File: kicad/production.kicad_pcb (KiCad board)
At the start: 2 copper layers, 76.2 x 78.7 mm, 54 parts, among them J1 ZX62R-B-5P, P1 CONN, SW1 RESET, SW2 IO0, U1 ESP-WROOM-32, U2 NJM2884, U3 FT231XS

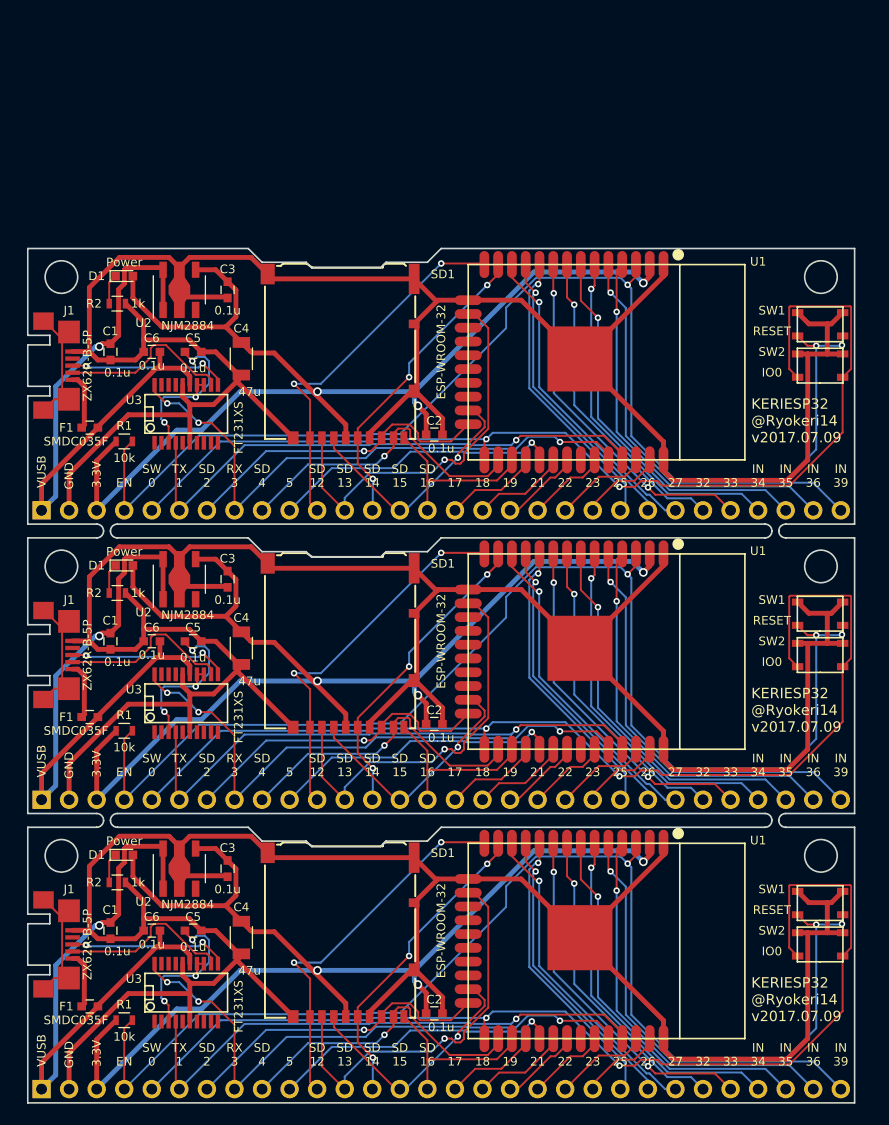
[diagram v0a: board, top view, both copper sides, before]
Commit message: 4枚面付け基板作成
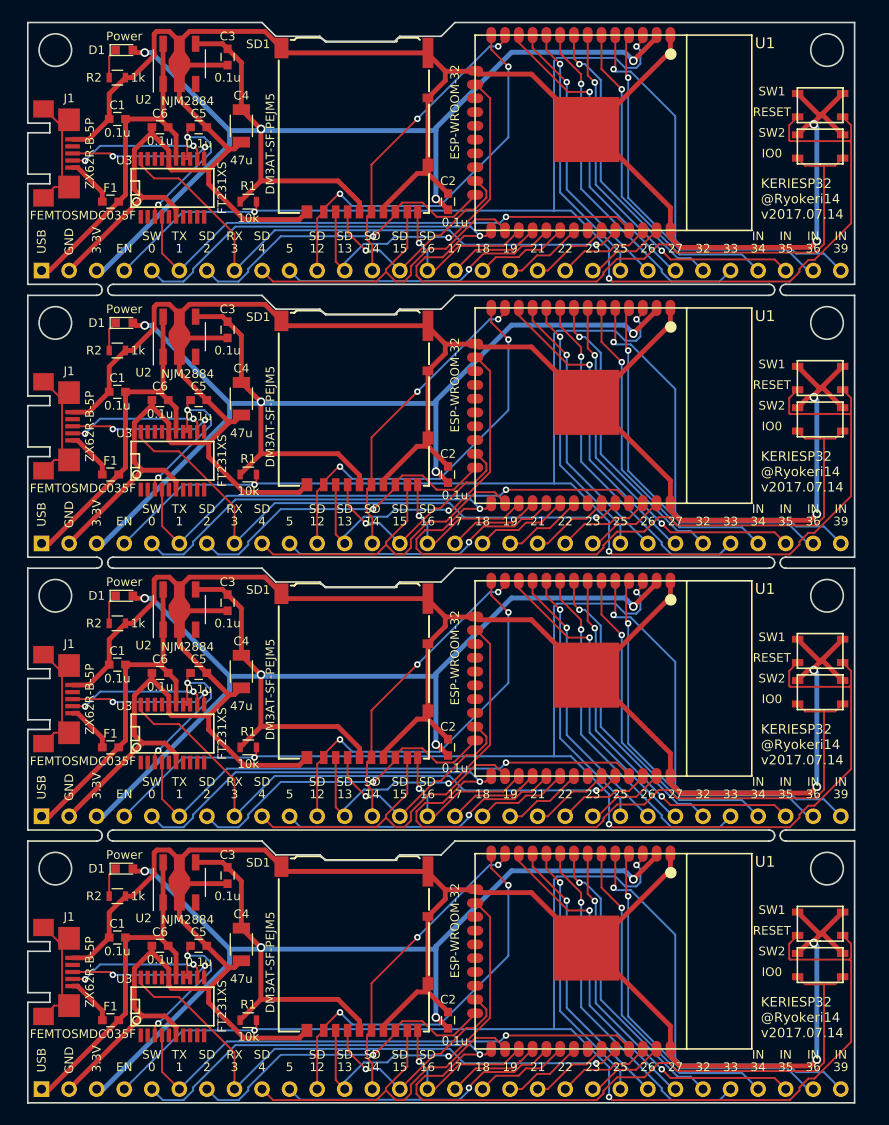
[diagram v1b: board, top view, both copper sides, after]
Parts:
- removed the C1 at (127.0, 51.4)
- removed the C1 at (127.0, 78.1)
- removed the C2 at (156.8, 59.1)
- removed the C2 at (156.8, 85.7)
- removed the C3 at (137.8, 45.7)
- removed the C3 at (137.8, 72.4)
- removed the C4 at (139.1, 52.1)
- removed the C4 at (139.1, 78.7)
- removed the C5 at (134.6, 51.4)
- removed the C5 at (134.6, 78.1)
- removed the C6 at (130.8, 51.4)
- removed the C6 at (130.8, 78.1)
- removed the D1 at (128.3, 44.5)
- removed the D1 at (128.3, 71.1)
- removed the F1 at (125.1, 58.4)
- removed the F1 at (125.1, 85.1)
- removed the J1 at (119.4, 52.7)
- removed the J1 at (119.4, 79.4)
- removed the P1 at (120.7, 92.7)
- removed the P1 at (120.7, 66.0)
- removed the R1 at (128.3, 59.7)
- removed the R1 at (128.3, 86.4)
- removed the R2 at (127.6, 47.0)
- removed the R2 at (127.6, 73.7)
- removed the SD1 at (148.6, 41.9)
- removed the SD1 at (148.6, 68.6)
- removed the SW1 at (192.4, 48.9)
- removed the SW1 at (192.4, 75.6)
- removed the SW2 at (192.4, 52.7)
- removed the SW2 at (192.4, 79.4)
- removed the U1 at (172.7, 52.4)
- removed the U1 at (172.7, 79.1)
- removed the U2 at (133.3, 45.7)
- removed the U2 at (133.3, 72.4)
- removed the U3 at (134.0, 57.1)
- removed the U3 at (134.0, 83.8)
- added C1: 0.1u, Capacitors_SMD:C_0603, F.Cu at (127.6, 30.0)
- added C1: 0.1u, Capacitors_SMD:C_0603, F.Cu at (127.6, 55.1)
- added C1: 0.1u, Capacitors_SMD:C_0603, F.Cu at (127.6, 80.3)
- added C2: 0.1u, Capacitors_SMD:C_0603, F.Cu at (158.1, 37.6)
- added C2: 0.1u, Capacitors_SMD:C_0603, F.Cu at (158.1, 62.7)
- added C2: 0.1u, Capacitors_SMD:C_0603, F.Cu at (158.1, 87.9)
- added C3: 0.1u, Capacitors_SMD:C_0603, F.Cu at (137.8, 24.3)
- added C3: 0.1u, Capacitors_SMD:C_0603, F.Cu at (137.8, 49.4)
- added C3: 0.1u, Capacitors_SMD:C_0603, F.Cu at (137.8, 74.5)
- added C4: 47u, Capacitors_SMD:C_1206, F.Cu at (139.1, 30.6)
- added C4: 47u, Capacitors_SMD:C_1206, F.Cu at (139.1, 55.8)
- added C4: 47u, Capacitors_SMD:C_1206, F.Cu at (139.1, 80.9)
- added C5: 0.1u, Capacitors_SMD:C_0603, F.Cu at (135.1, 30.7)
- added C5: 0.1u, Capacitors_SMD:C_0603, F.Cu at (135.1, 55.9)
- added C5: 0.1u, Capacitors_SMD:C_0603, F.Cu at (135.1, 81.0)
- added C6: 0.1u, Capacitors_SMD:C_0603, F.Cu at (131.6, 30.7)
- added C6: 0.1u, Capacitors_SMD:C_0603, F.Cu at (131.6, 55.9)
- added C6: 0.1u, Capacitors_SMD:C_0603, F.Cu at (131.6, 81.0)
- added D1: Power, LEDs:LED_0603, F.Cu at (128.3, 23.6)
- added D1: Power, LEDs:LED_0603, F.Cu at (128.3, 48.8)
- added D1: Power, LEDs:LED_0603, F.Cu at (128.3, 73.9)
- added F1: FEMTOSMDC035F, Capacitors_SMD:C_0603, F.Cu at (127.0, 37.6)
- added F1: FEMTOSMDC035F, Capacitors_SMD:C_0603, F.Cu at (127.0, 62.7)
- added F1: FEMTOSMDC035F, Capacitors_SMD:C_0603, F.Cu at (127.0, 87.9)
- added J1: ZX62R-B-5P, KERIESP32:ZX62R-B-5P, F.Cu at (119.4, 33.1)
- added J1: ZX62R-B-5P, KERIESP32:ZX62R-B-5P, F.Cu at (119.4, 58.3)
- added J1: ZX62R-B-5P, KERIESP32:ZX62R-B-5P, F.Cu at (119.4, 83.4)
- added P1: CONN, KERIESP32:Pin_Header_Straight_1x30_Pitch2.54mm, B.Cu at (120.7, 43.9)
- added P1: CONN, KERIESP32:Pin_Header_Straight_1x30_Pitch2.54mm, B.Cu at (120.7, 69.1)
- added P1: CONN, KERIESP32:Pin_Header_Straight_1x30_Pitch2.54mm, B.Cu at (120.7, 94.2)
- added R1: 10k, Resistors_SMD:R_0603, F.Cu at (139.7, 37.6)
- added R1: 10k, Resistors_SMD:R_0603, F.Cu at (139.7, 62.7)
- added R1: 10k, Resistors_SMD:R_0603, F.Cu at (139.7, 87.9)
- added R2: 1k, Resistors_SMD:R_0603, F.Cu at (127.6, 26.2)
- added R2: 1k, Resistors_SMD:R_0603, F.Cu at (127.6, 51.3)
- added R2: 1k, Resistors_SMD:R_0603, F.Cu at (127.6, 76.5)
- added SD1: DM3AT-SF-PEJM5, KERIESP32:HIROSE-MICROSD-DM3AT-SF, F.Cu at (149.9, 21.1)
- added SD1: DM3AT-SF-PEJM5, KERIESP32:HIROSE-MICROSD-DM3AT-SF, F.Cu at (149.9, 46.2)
- added SD1: DM3AT-SF-PEJM5, KERIESP32:HIROSE-MICROSD-DM3AT-SF, F.Cu at (149.9, 71.4)
- added SW1: RESET, KERIESP32:SW_PUSH, F.Cu at (192.4, 28.7)
- added SW1: RESET, KERIESP32:SW_PUSH, F.Cu at (192.4, 53.8)
- added SW1: RESET, KERIESP32:SW_PUSH, F.Cu at (192.4, 79.0)
- added SW2: IO0, KERIESP32:SW_PUSH, F.Cu at (192.4, 32.5)
- added SW2: IO0, KERIESP32:SW_PUSH, F.Cu at (192.4, 57.7)
- added SW2: IO0, KERIESP32:SW_PUSH, F.Cu at (192.4, 82.8)
- added U1: ESP-WROOM-32, KERIESP32:ESP-WROOM-32, F.Cu at (173.4, 31.2)
- added U1: ESP-WROOM-32, KERIESP32:ESP-WROOM-32, F.Cu at (173.4, 56.4)
- added U1: ESP-WROOM-32, KERIESP32:ESP-WROOM-32, F.Cu at (173.4, 81.5)
- added U2: NJM2884, TO_SOT_Packages_SMD:SOT89-5_Housing, F.Cu at (133.3, 24.9)
- added U2: NJM2884, TO_SOT_Packages_SMD:SOT89-5_Housing, F.Cu at (133.3, 50.0)
- added U2: NJM2884, TO_SOT_Packages_SMD:SOT89-5_Housing, F.Cu at (133.3, 75.2)
- added U3: FT231XS, SMD_Packages:SSOP-20, F.Cu at (132.7, 36.3)
- added U3: FT231XS, SMD_Packages:SSOP-20, F.Cu at (132.7, 61.5)
- added U3: FT231XS, SMD_Packages:SSOP-20, F.Cu at (132.7, 86.6)
- F1: value SMDC035F -> FEMTOSMDC035F
- P1: footprint Pin_Headers:Pin_Header_Straight_1x30_Pitch2.54mm -> KERIESP32:Pin_Header_Straight_1x30_Pitch2.54mm
- SD1: value Micro_SD -> DM3AT-SF-PEJM5
- moved R1 11.4 mm to (139.7, 113.0)
- moved J1 2.54 mm to (119.4, 108.6)
- moved F1 2.29 mm to (127.0, 113.0)
- moved SW1 1.91 mm to (192.4, 104.1)
- moved SW2 1.91 mm to (192.4, 108.0)
- moved U3 1.80 mm to (132.7, 111.8)
- moved SD1 1.80 mm to (149.9, 96.5)
- moved C6 1.59 mm to (131.6, 106.2)
- moved C5 1.49 mm to (135.1, 106.2)
- moved C2 1.42 mm to (158.1, 113.0), turned to 90 degrees
- moved D1 1.27 mm to (128.3, 99.1)
- moved R2 1.27 mm to (127.6, 101.6)
- moved U2 1.27 mm to (133.3, 100.3)
- moved U1 1.14 mm to (173.4, 106.7)
- moved C1 0.90 mm to (127.6, 105.4), turned to 180 degrees
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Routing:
- net GND: track 617.2 -> 799.9 mm, vias 0 -> 8
- net ENABLE: track 342.9 -> 483.0 mm, vias 9 -> 12
- net +3V3: track 328.8 -> 449.3 mm, vias 9 -> 16
- net IO0: track 292.5 -> 377.2 mm, vias 6 -> 4
- net RXD: track 163.7 -> 211.9 mm, vias 9 -> 4
- net SD_SD1: track 86.2 -> 132.8 mm, vias 3 -> 0
- net TXD: track 154.0 -> 198.7 mm, vias 3 -> 4
- net SD_SD2: track 104.1 -> 146.8 mm, vias 6 -> 8
- net +5V: track 169.8 -> 128.5 mm, vias 3 -> 0
- net Net-(P1-Pad30): track 117.3 -> 154.1 mm, vias 3 -> 4
- net Net-(P1-Pad26): track 97.9 -> 131.3 mm, vias 6 -> 4
- net Net-(P1-Pad28): track 106.9 -> 139.5 mm, vias 3 -> 8
- net SD_SD0: track 87.9 -> 120.1 mm, vias 3 -> 4
- net Net-(P1-Pad29): track 110.2 -> 140.1 mm, vias 3 -> 4
- net Net-(P1-Pad24): track 89.2 -> 115.9 mm, vias 3 -> 4
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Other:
- board size 76.2 x 78.7 mm -> 76.2 x 99.6 mm
- board text added: "KERIESP32 @Ryokeri14 v2017.07.14"
- board text added: "USB"
- board text removed: "KERIESP32 @Ryokeri14 v2017.07.09"
- board text removed: "VUSB"
